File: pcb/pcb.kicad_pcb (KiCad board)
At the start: 2 copper layers, 118.8 x 99.7 mm, 86 parts

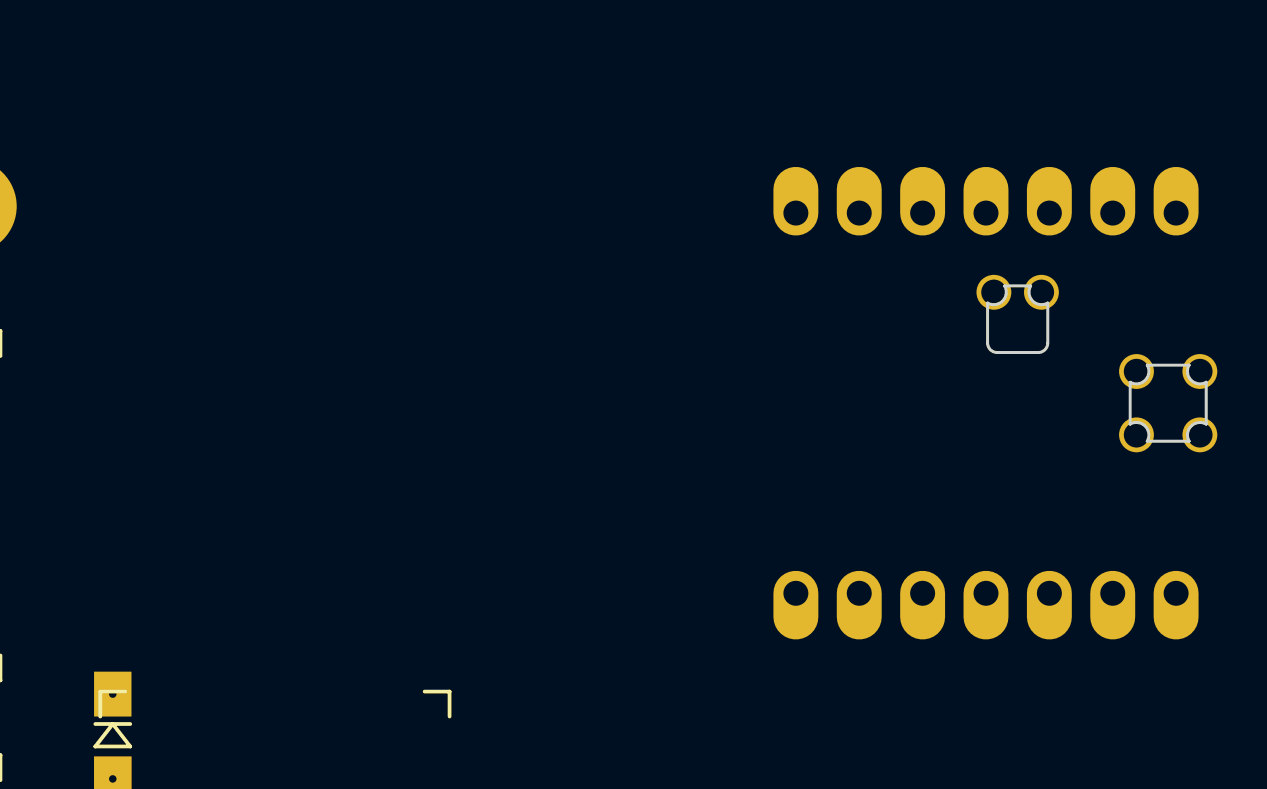
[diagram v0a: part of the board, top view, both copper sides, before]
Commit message: Update placement
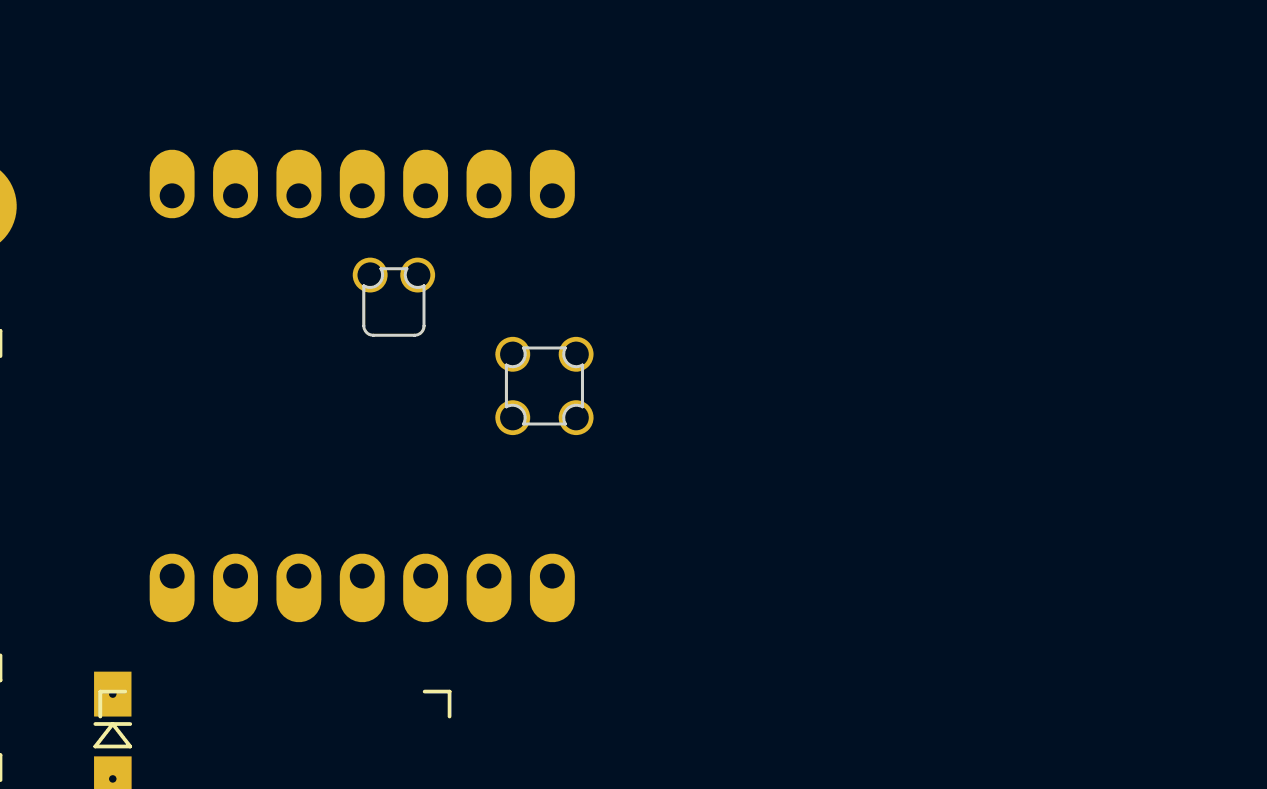
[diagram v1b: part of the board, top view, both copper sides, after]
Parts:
- moved MCUR1 25.0 mm to (263.5, 39.7)
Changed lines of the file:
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@@
 		(legacy_teardrops no)
 	)
-	(paper "User" 500 200)
+	(paper "User" 300 200)
 	(title_block
 		(title "Charma Wireless Split Keyboard")
@@
 	(footprint "charmalib:XIAO_nRF52840_SMD_Cutout"
 		(layer "F.Cu")
-		(at 288.5 40.39 -90)
+		(at 263.5 39.7 -90)
 		(property "Reference" "MCUR1"
 			(at -19.3989 -11.28268 90)
